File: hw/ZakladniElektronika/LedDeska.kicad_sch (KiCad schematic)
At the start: 16 parts, among them U1 LDC1314

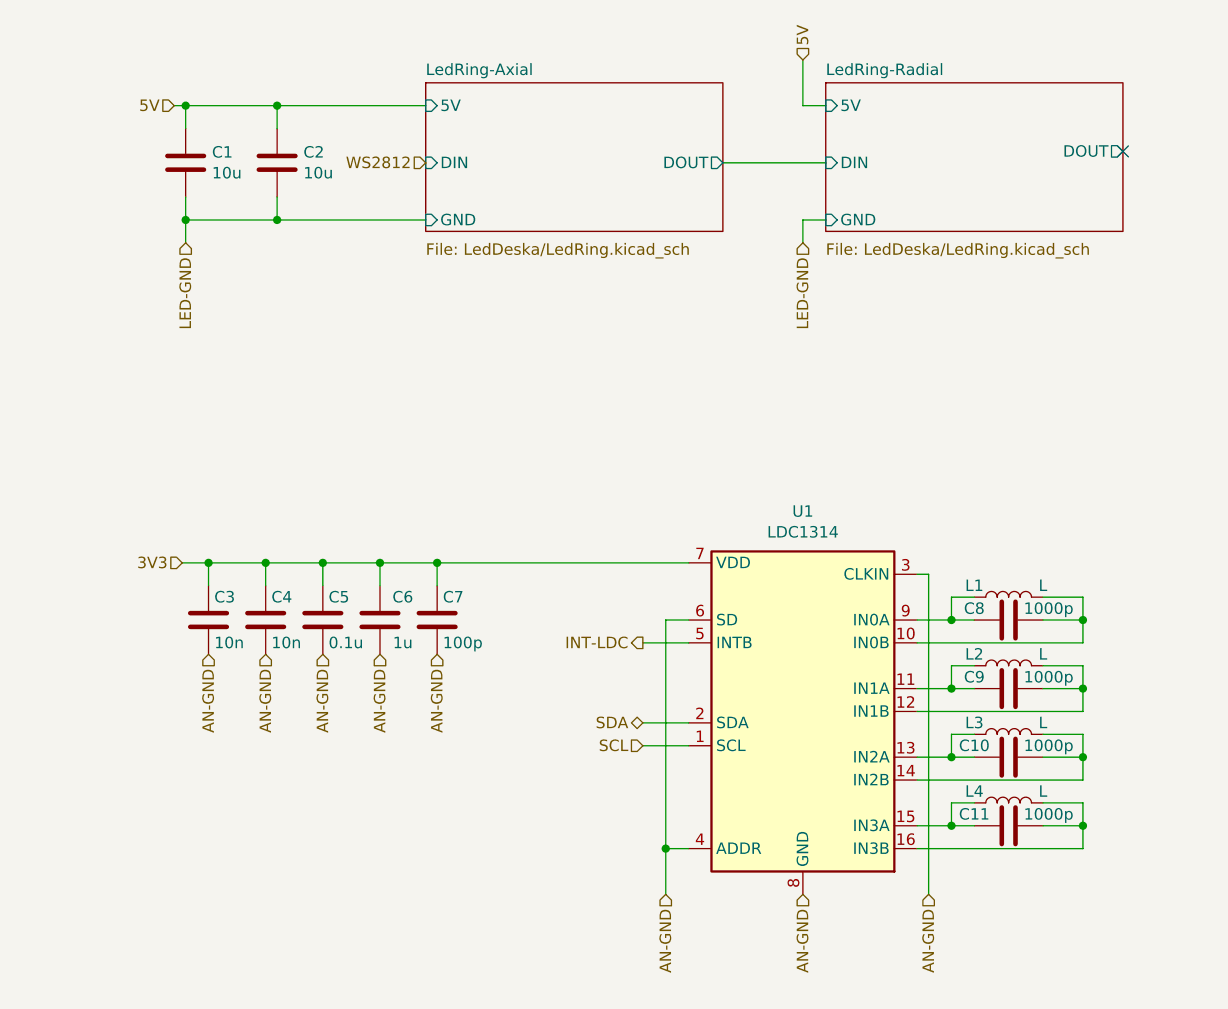
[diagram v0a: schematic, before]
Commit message: WIP
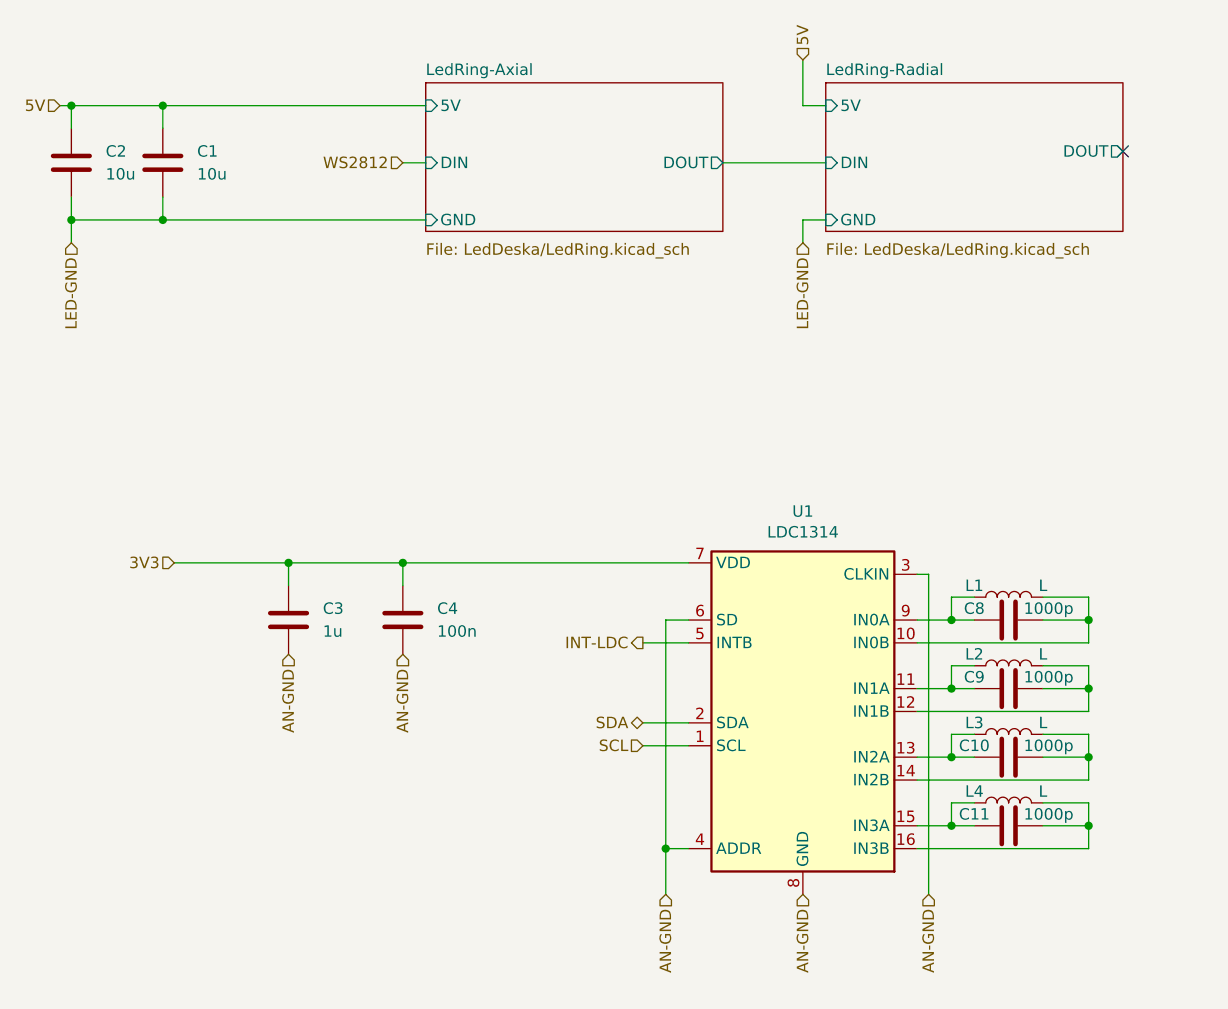
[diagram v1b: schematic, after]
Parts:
- removed C1, C2: 10u, Capacitor_SMD:C_0805_2012Metric, symbol B.B-rescue:C-Device-B.B-rescue
- removed C3, C4: 10n, Capacitor_SMD:C_0402_1005Metric, symbol B.B-rescue:C-Device-B.B-rescue
- removed C5: 0.1u, Resistor_SMD:R_0402_1005Metric, symbol B.B-rescue:C-Device-B.B-rescue
- removed C6: 1u, Capacitor_SMD:C_0402_1005Metric, symbol B.B-rescue:C-Device-B.B-rescue
- removed C7: 100p, Capacitor_SMD:C_0402_1005Metric, symbol B.B-rescue:C-Device-B.B-rescue
- added C1, C2: 10u, Capacitor_SMD:C_0805_2012Metric, symbol Device:C
- added C3: 1u, Capacitor_SMD:C_0402_1005Metric, symbol Device:C
- added C4: 100n, Capacitor_SMD:C_0402_1005Metric, symbol Device:C
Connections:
- net 3V3: now also C3.1, C4.1
- net 5V: now also C1.1, C2.1
- net AN-GND: now also C3.2, C4.2
- net LED-GND: now also C1.2, C2.2

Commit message: WIP
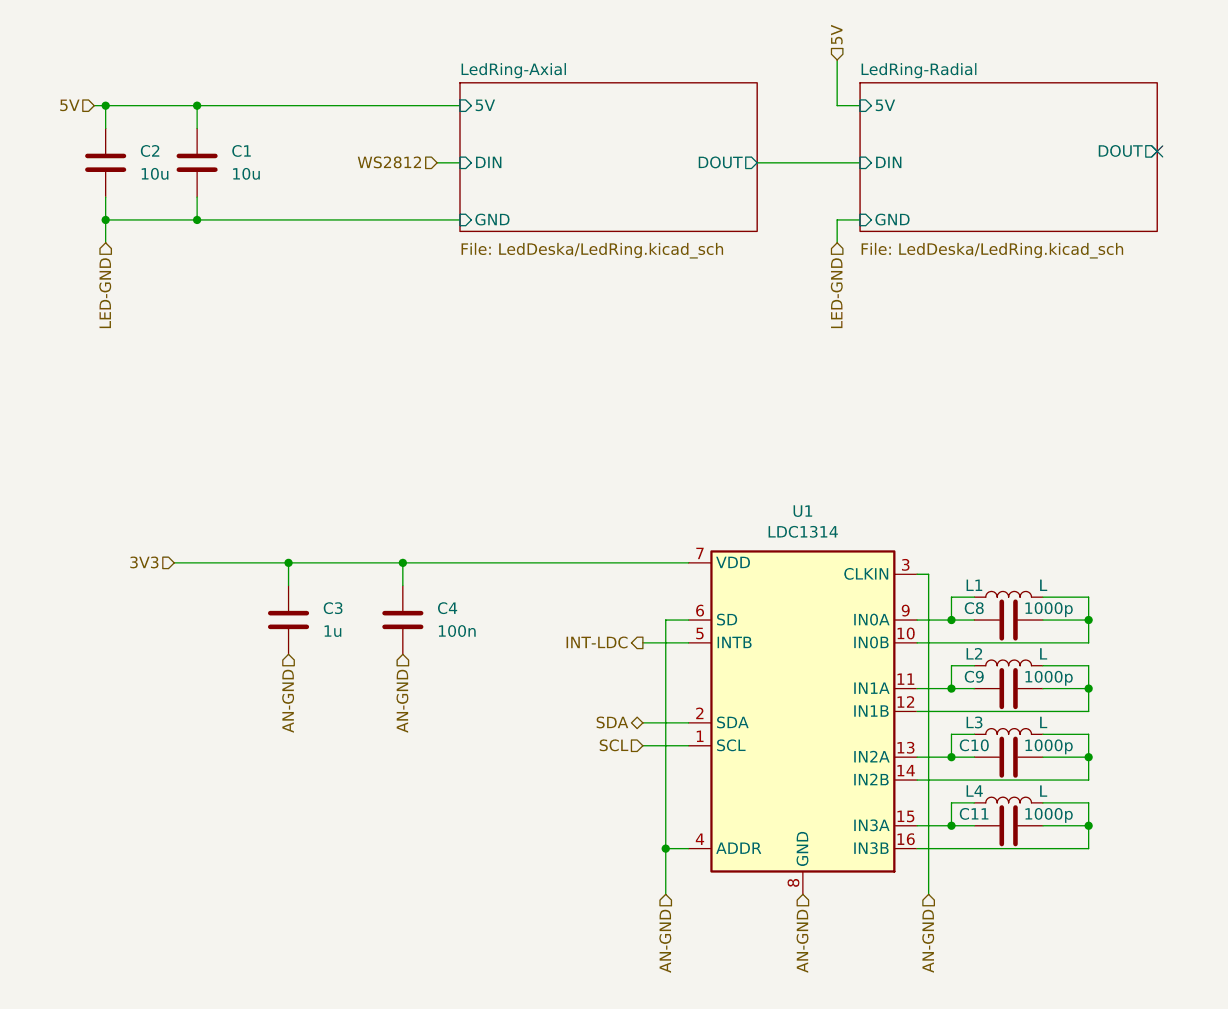
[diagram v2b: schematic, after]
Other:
- moved on the sheet: C1, C2
